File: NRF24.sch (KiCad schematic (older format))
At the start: 46 parts, among them J1 Conn_ARM_JTAG_SWD_10, J2 SMA, Q1 AO3401A, Q2 AO3401A, Q3 AO3401A, U1 SHT21, U2 STM32L031G6Ux, U3 nRF24L01P, Y1 16MHz

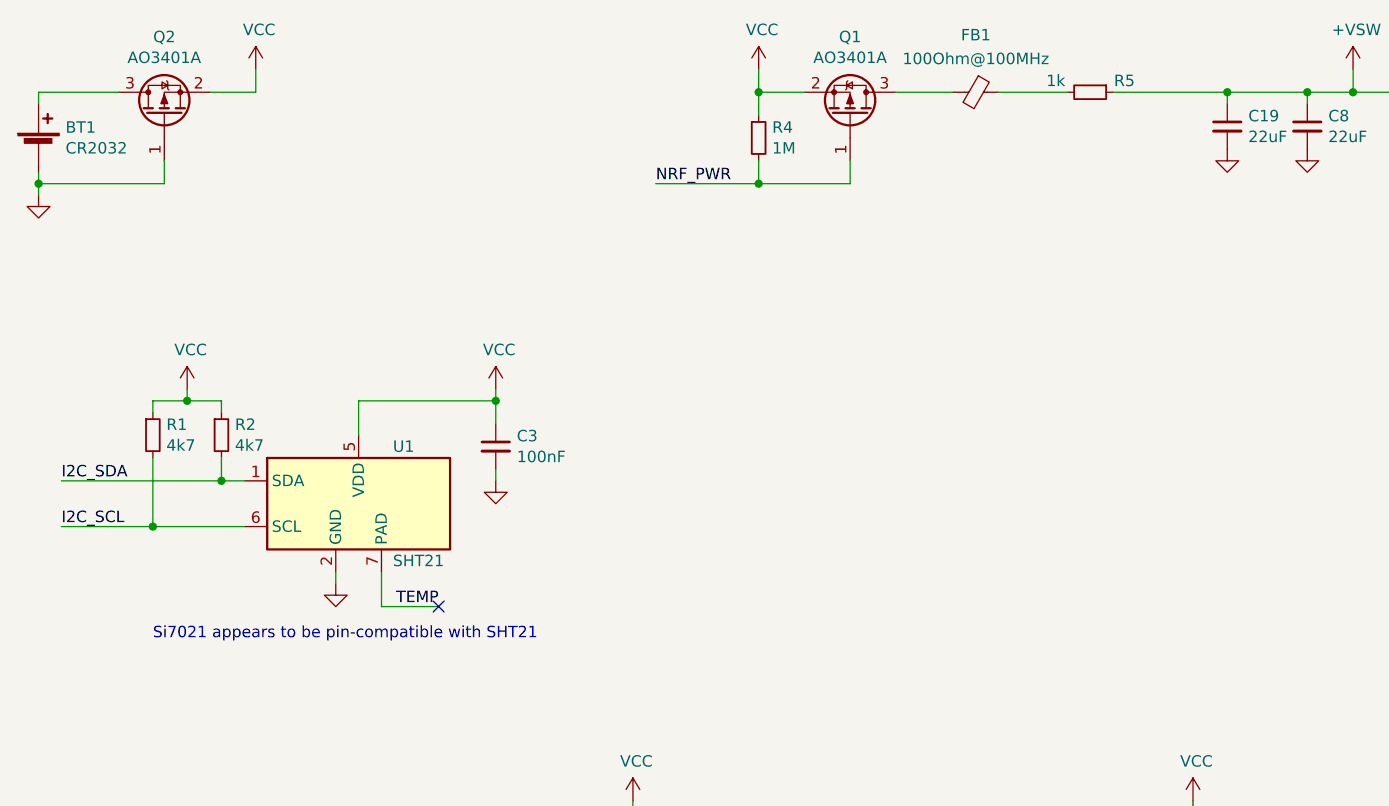
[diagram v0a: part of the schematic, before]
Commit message: Minor changes
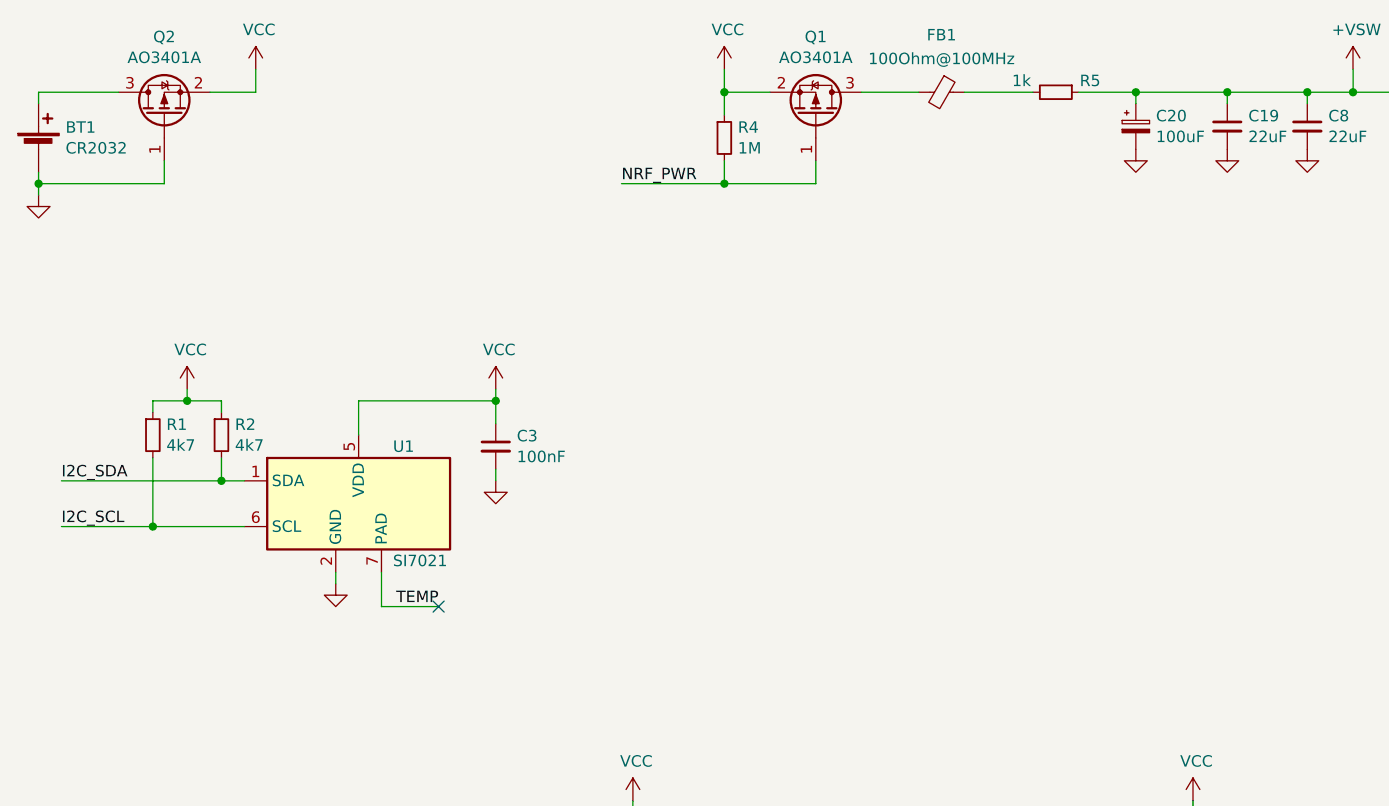
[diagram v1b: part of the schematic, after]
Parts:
- added C20: 100uF, Capacitor_Tantalum_SMD:CP_EIA-3528-15_AVX-H, symbol Device:CP_Small
- U1: value SHT21 -> SI7021; LCSC C84828 -> C132603
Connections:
- net +VSW: now also C20.1
- net GND: now also C20.2
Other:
- note removed: "Si7021 appears to be pin-compatible with SHT21"
- moved on the sheet: FB1, Q1, R4, R5
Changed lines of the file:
@@
 L Device:R_Small R5
 U 1 1 5F6EDFC5
-P 5500 1050
-F 0 "R5" V 5450 1200 50  0000 C CNN
-F 1 "1k" V 5450 900 50  0000 C CNN
-F 2 "Resistor_SMD:R_0402_1005Metric" H 5500 1050 50  0001 C CNN
-F 3 "~" H 5500 1050 50  0001 C CNN
-F 4 "C11702" H 5500 1050 50  0001 C CNN "LCSC"
-	1    5500 1050
+P 5350 1050
+F 0 "R5" V 5300 1200 50  0000 C CNN
+F 1 "1k" V 5300 900 50  0000 C CNN
+F 2 "Resistor_SMD:R_0402_1005Metric" H 5350 1050 50  0001 C CNN
+F 3 "~" H 5350 1050 50  0001 C CNN
+F 4 "C11702" H 5350 1050 50  0001 C CNN "LCSC"
+	1    5350 1050
 	0    1    1    0
 $EndComp
 Wire Wire Line
-	4650 1050 4900 1050
+	4500 1050 4750 1050
 Wire Wire Line
 	8150 1050 8250 1050
@@
 L Device:R_Small R4
 U 1 1 5F6FC380
-P 4050 1250
-F 0 "R4" H 4109 1296 50  0000 L CNN
-F 1 "1M" H 4109 1205 50  0000 L CNN
-F 2 "Resistor_SMD:R_0402_1005Metric" H 4050 1250 50  0001 C CNN
-F 3 "~" H 4050 1250 50  0001 C CNN
-F 4 "C26083" H 4050 1250 50  0001 C CNN "LCSC"
-	1    4050 1250
-	1    0    0    -1
-$EndComp
-Wire Wire Line
-	4050 1150 4050 1050
-Wire Wire Line
-	4050 1050 4250 1050
-Wire Wire Line
-	4050 1350 4050 1450
-Wire Wire Line
-	4450 1450 4450 1350
+P 3900 1250
+F 0 "R4" H 3959 1296 50  0000 L CNN
+F 1 "1M" H 3959 1205 50  0000 L CNN
+F 2 "Resistor_SMD:R_0402_1005Metric" H 3900 1250 50  0001 C CNN
+F 3 "~" H 3900 1250 50  0001 C CNN
+F 4 "C26083" H 3900 1250 50  0001 C CNN "LCSC"
+	1    3900 1250
+	1    0    0    -1
+$EndComp
+Wire Wire Line
+	3900 1150 3900 1050
+Wire Wire Line
+	3900 1050 4100 1050
+Wire Wire Line
+	3900 1350 3900 1450
+Wire Wire Line
+	4300 1450 4300 1350
 Wire Wire Line
 	5000 4550 5100 4550
@@
 	5000 4550 5000 4600
 Wire Wire Line
-	4050 1450 4450 1450
+	3900 1450 4300 1450
 Wire Wire Line
 	1900 4800 2350 4800
@@
 P 2300 2850
 F 0 "U1" H 2450 3100 50  0000 L CNN
-F 1 "SHT21" H 2450 2600 50  0000 L CNN
+F 1 "SI7021" H 2450 2600 50  0000 L CNN
 F 2 "Package_DFN_QFN:DFN-6-1EP_3x3mm_P1mm_EP1.5x2.4mm" H 2300 2450 50  0001 C CNN
 F 3 "https://www.silabs.com/documents/public/data-sheets/Si7021-A20.pdf" H 2100 3150 50  0001 C CNN
-F 4 "C84828" H 2300 2850 50  0001 C CNN "LCSC"
+F 4 "C132603" H 2300 2850 50  0001 C CNN "LCSC"
 	1    2300 2850
 	1    0    0    -1
@@
 	1350 5750 1400 5750
 Wire Wire Line
-	4050 950  4050 1050
-Connection ~ 4050 1050
+	3900 950  3900 1050
+Connection ~ 3900 1050
 Connection ~ 6450 1050
 Wire Wire Line
@@
 	6450 1050 6450 1100
 Wire Wire Line
-	5600 1050 6100 1050
+	5450 1050 5700 1050
 $Comp
 L Device:C_Small C8
@@
 $EndComp
 Wire Wire Line
-	4050 1450 3600 1450
-Connection ~ 4050 1450
+	3900 1450 3450 1450
+Connection ~ 3900 1450
 Connection ~ 2900 2400
 Wire Wire Line
@@
 Wire Wire Line
 	7800 5800 7800 5850
-Text Label 3600 1450 0    50   ~ 0
+Text Label 3450 1450 0    50   ~ 0
 NRF_PWR
 Wire Wire Line
@@
 L power:VCC #PWR016
 U 1 1 5F79FBFF
-P 4050 950
-F 0 "#PWR016" H 4050 800 50  0001 C CNN
-F 1 "VCC" H 4065 1123 50  0000 C CNN
-F 2 "" H 4050 950 50  0001 C CNN
-F 3 "" H 4050 950 50  0001 C CNN
-	1    4050 950
+P 3900 950
+F 0 "#PWR016" H 3900 800 50  0001 C CNN
+F 1 "VCC" H 3915 1123 50  0000 C CNN
+F 2 "" H 3900 950 50  0001 C CNN
+F 3 "" H 3900 950 50  0001 C CNN
+	1    3900 950
 	1    0    0    -1
 $EndComp
@@
 L Device:Ferrite_Bead_Small FB1
 U 1 1 5F7E119C
-P 5000 1050
-F 0 "FB1" V 4750 1050 50  0000 C CNN
-F 1 "100Ohm@100MHz" V 4854 1050 50  0000 C CNN
-F 2 "Inductor_SMD:L_0805_2012Metric" V 4930 1050 50  0001 C CNN
-F 3 "~" H 5000 1050 50  0001 C CNN
-F 4 "C1015" H 5000 1050 50  0001 C CNN "LCSC"
-	1    5000 1050
+P 4850 1050
+F 0 "FB1" V 4600 1050 50  0000 C CNN
+F 1 "100Ohm@100MHz" V 4704 1050 50  0000 C CNN
+F 2 "Inductor_SMD:L_0805_2012Metric" V 4780 1050 50  0001 C CNN
+F 3 "~" H 4850 1050 50  0001 C CNN
+F 4 "C1015" H 4850 1050 50  0001 C CNN "LCSC"
+	1    4850 1050
 	0    1    1    0
 $EndComp
 Wire Wire Line
-	5100 1050 5400 1050
+	4950 1050 5250 1050
 $Comp
 L power:PWR_FLAG #FLG0103
@@
 L Transistor_FET:AO3401A Q1
 U 1 1 5F790A3D
-P 4450 1150
-F 0 "Q1" V 4792 1150 50  0000 C CNN
-F 1 "AO3401A" V 4701 1150 50  0000 C CNN
-F 2 "Package_TO_SOT_SMD:SOT-23" H 4650 1075 50  0001 L CIN
-F 3 "http://www.aosmd.com/pdfs/datasheet/AO3401A.pdf" H 4450 1150 50  0001 L CNN
-F 4 "C15127" V 4450 1150 50  0001 C CNN "LCSC"
-	1    4450 1150
+P 4300 1150
+F 0 "Q1" V 4642 1150 50  0000 C CNN
+F 1 "AO3401A" V 4551 1150 50  0000 C CNN
+F 2 "Package_TO_SOT_SMD:SOT-23" H 4500 1075 50  0001 L CIN
+F 3 "http://www.aosmd.com/pdfs/datasheet/AO3401A.pdf" H 4300 1150 50  0001 L CNN
+F 4 "C15127" V 4300 1150 50  0001 C CNN "LCSC"
+	1    4300 1150
 	0    1    -1   0
 $EndComp
@@
 Wire Wire Line
 	8950 6100 8800 6100
-Text Notes 1400 3450 0    50   ~ 0
-Si7021 appears to be pin-compatible with SHT21
+$Comp
+L Device:CP_Small C20
+U 1 1 5F834F56
+P 5700 1200
+F 0 "C20" H 5788 1246 50  0000 L CNN
+F 1 "100uF" H 5788 1155 50  0000 L CNN
+F 2 "Capacitor_Tantalum_SMD:CP_EIA-3528-15_AVX-H" H 5700 1200 50  0001 C CNN
+F 3 "~" H 5700 1200 50  0001 C CNN
+F 4 "C16133" H 5700 1200 50  0001 C CNN "LCSC"
+	1    5700 1200
+	1    0    0    -1
+$EndComp
+Wire Wire Line
+	5700 1100 5700 1050
+Connection ~ 5700 1050
+Wire Wire Line
+	5700 1050 6100 1050
+$Comp
+L power:GND #PWR031
+U 1 1 5F843526
+P 5700 1300
+F 0 "#PWR031" H 5700 1050 50  0001 C CNN
+F 1 "GND" H 5705 1127 50  0001 C CNN
+F 2 "" H 5700 1300 50  0001 C CNN
+F 3 "" H 5700 1300 50  0001 C CNN
+	1    5700 1300
+	1    0    0    -1
+$EndComp
 $EndSCHEMATC
